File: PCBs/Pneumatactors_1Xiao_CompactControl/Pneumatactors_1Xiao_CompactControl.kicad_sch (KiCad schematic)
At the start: 20 parts, among them J1 Valve_1, J2 Valve_2, J3 Pump, J4 Pogo Connection, Q1 IRLML2060, Q2 IRLML2060, U1 SeeeduinoXIAO, U2 Pololu 2990, U3 TS01AQE

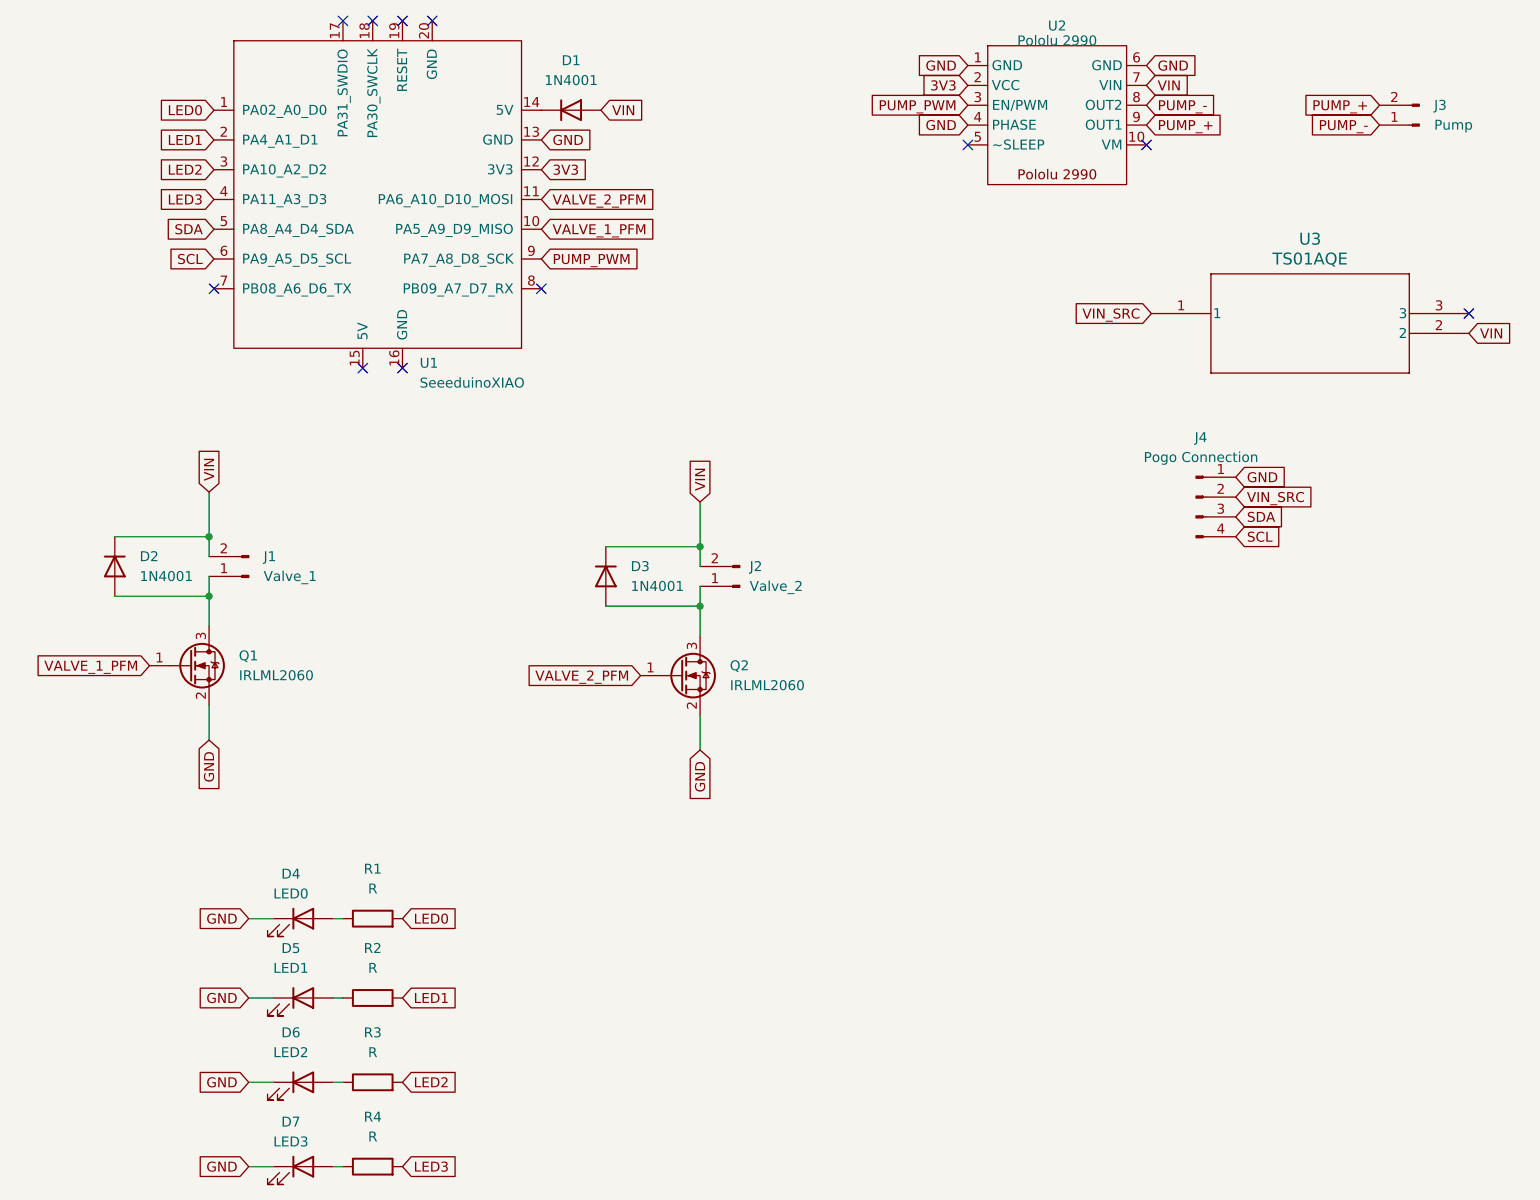
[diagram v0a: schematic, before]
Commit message: 2025-03-24 00:00:04
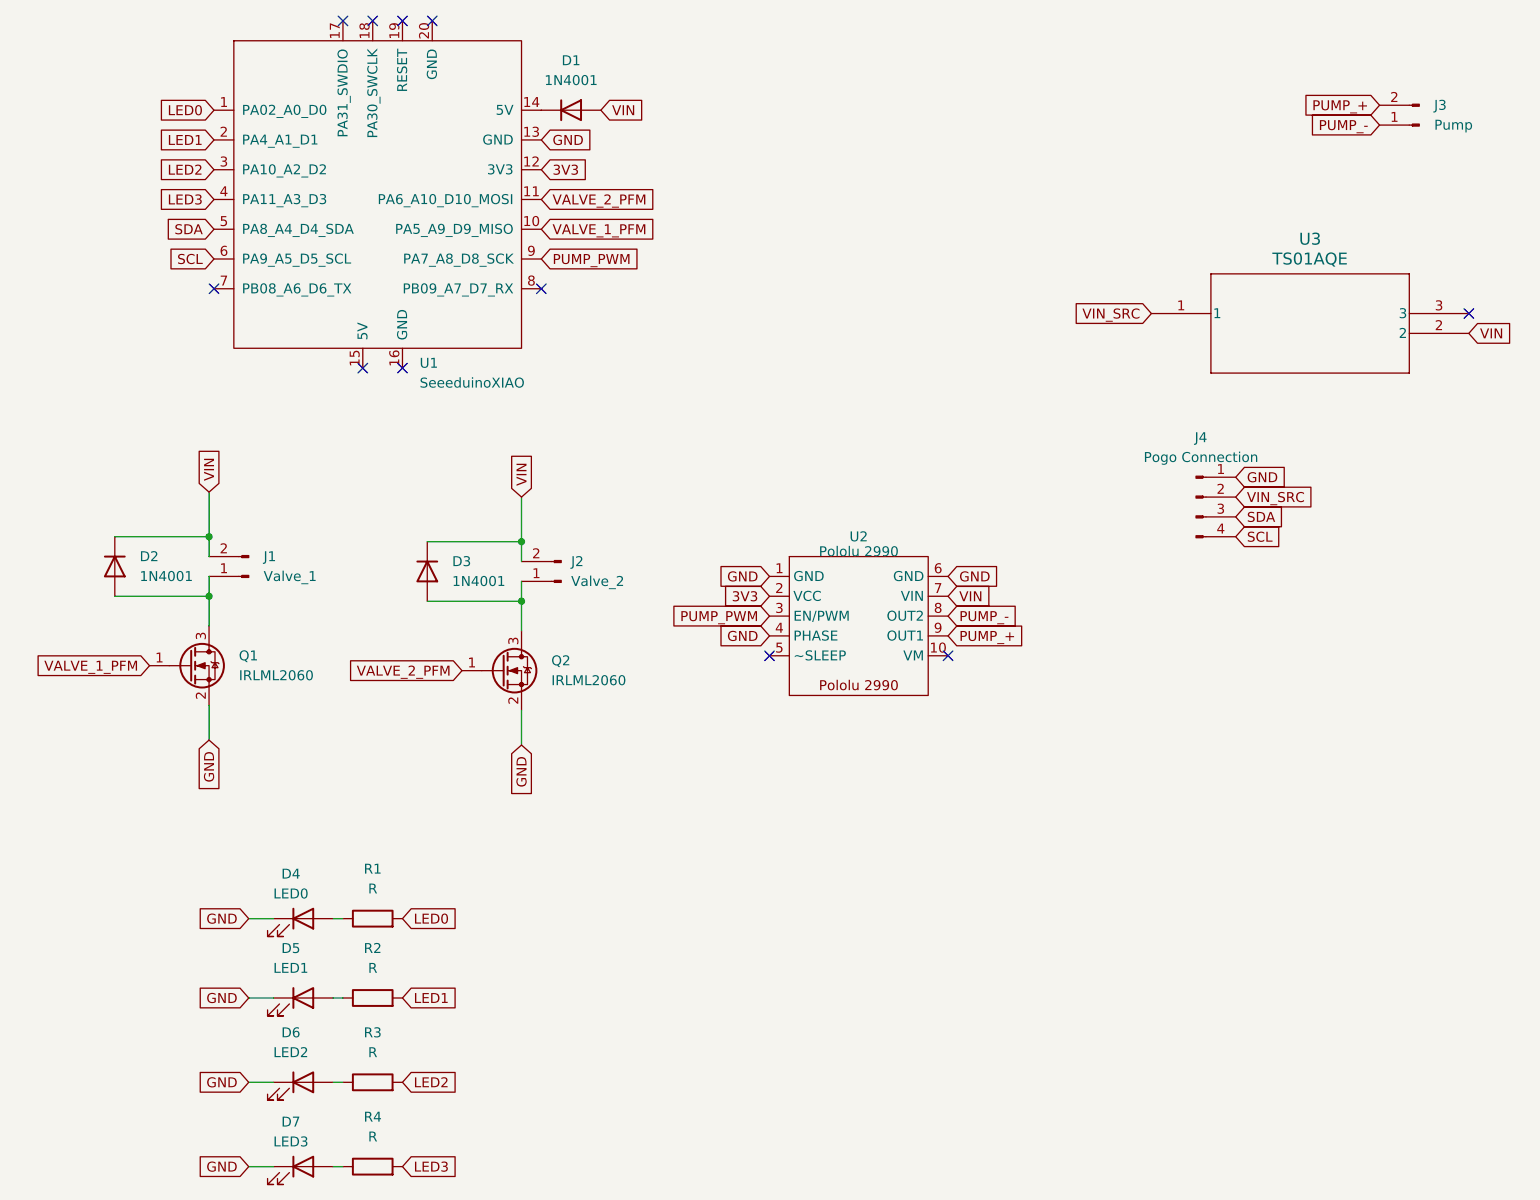
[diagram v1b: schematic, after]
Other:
- moved on the sheet: D3, J2, Q2, U2
